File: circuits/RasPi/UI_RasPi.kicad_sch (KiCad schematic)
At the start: 14 parts, among them Q30 BSS138, Q33 BSS138

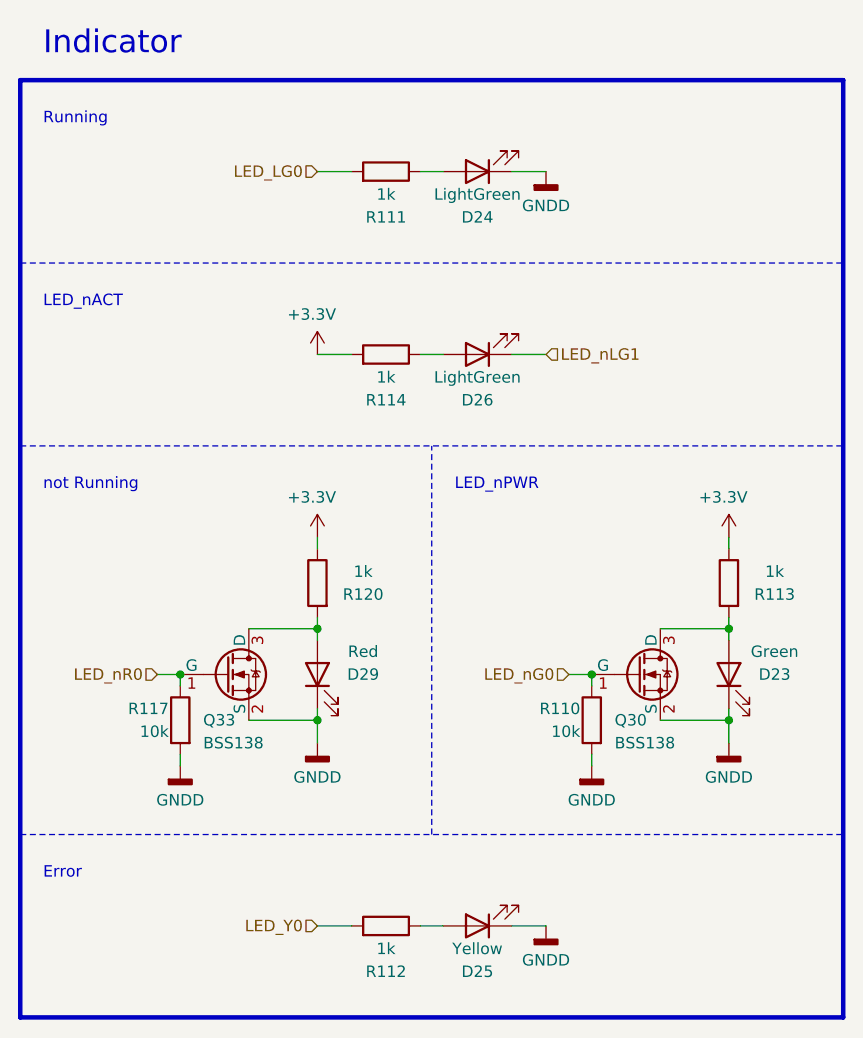
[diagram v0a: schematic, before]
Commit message: 更新
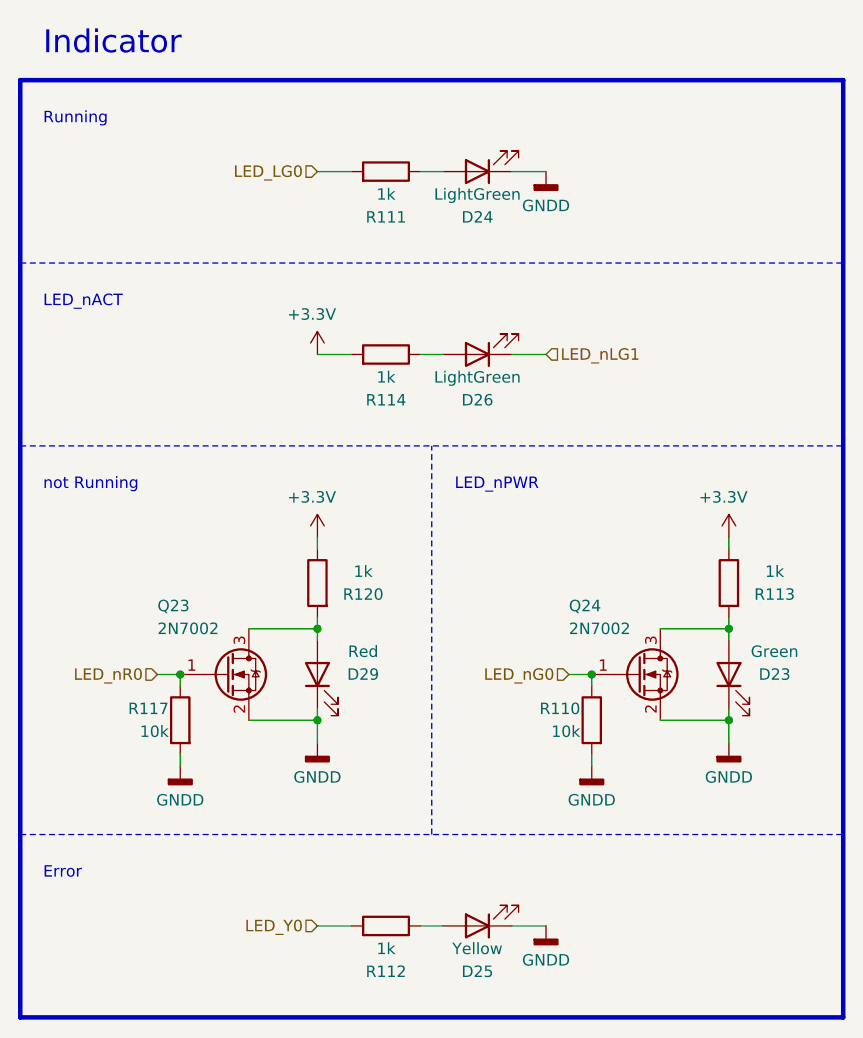
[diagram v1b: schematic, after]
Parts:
- removed Q30, Q33: BSS138, Package_TO_SOT_SMD:SOT-23, symbol Device:Q_NMOS_GSD
- added Q23, Q24: 2N7002, Package_TO_SOT_SMD:SOT-23, symbol Transistor_FET:2N7002
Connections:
- net GNDD: now also Q23.2 (S), Q24.2 (S)
- net LED_nG0: now also Q24.1 (G)
- net LED_nR0: now also Q23.1 (G)
- net at D23.2 (A), R113.2: now also Q24.3 (D)
- net at D29.2 (A), R120.2: now also Q23.3 (D)
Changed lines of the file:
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@@
   (junction (at 147.32 106.68) (diameter 0) (color 0 0 0 0)
   )
+  (junction (at 132.08 111.76) (diameter 0) (color 0 0 0 0)
+  )
+  (junction (at 147.32 116.84) (diameter 0) (color 0 0 0 0)
+  )
   (junction (at 177.8 111.76) (diameter 0) (color 0 0 0 0)
-  )
-  (junction (at 147.32 116.84) (diameter 0) (color 0 0 0 0)
-  )
-  (junction (at 132.08 111.76) (diameter 0) (color 0 0 0 0)
   )
   (junction (at 193.04 116.84) (diameter 0) (color 0 0 0 0)
@@
     )
   )
+  (symbol (lib_id "Transistor_FET:2N7002") (at 137.16 111.76 0) (unit 1)
+    (in_bom yes) (on_board yes) (dnp no)
+    (property "Reference" "Q23" (at 129.54 104.14 0)
+      (effects (font (size 1.27 1.27)) (justify left))
+    )
+    (property "Value" "2N7002" (at 129.54 106.68 0)
+      (effects (font (size 1.27 1.27)) (justify left))
+    )
+    (property "Footprint" "Package_TO_SOT_SMD:SOT-23" (at 142.24 113.665 0)
+      (effects (font (size 1.27 1.27) italic) (justify left) hide)
+    )
+    (property "Datasheet" "https://www.onsemi.com/pub/Collateral/NDS7002A-D.PDF" (at 142.24 115.57 0)
+      (effects (font (size 1.27 1.27)) (justify left) hide)
+    )
+    (pin "3")
+    (pin "1")
+    (pin "2")
+    (instances
+      (project "RasPi"
+        (path "/689a9e74-f202-4ea4-bfbb-4341f2549250/fddad0c3-2af8-46e3-8794-fa1122d24d51/69fce92a-28f6-4191-9f2f-418081756bee"
+          (reference "Q23") (unit 1)
+        )
+      )
+    )
+  )
   (symbol (lib_id "Device:LED") (at 193.04 111.76 90) (unit 1)
     (in_bom yes) (on_board yes) (dnp no)
@@
         (path "/689a9e74-f202-4ea4-bfbb-4341f2549250/fddad0c3-2af8-46e3-8794-fa1122d24d51/69fce92a-28f6-4191-9f2f-418081756bee"
           (reference "R120") (unit 1)
-        )
-      )
-    )
-  )
-  (symbol (lib_name "Q_NMOS_GSD_1") (lib_id "Device:Q_NMOS_GSD") (at 182.88 111.76 0) (unit 1)
-    (in_bom yes) (on_board yes) (dnp no)
-    (property "Reference" "Q30" (at 180.34 116.84 0)
-      (effects (font (size 1.27 1.27)) (justify left))
-    )
-    (property "Value" "BSS138" (at 180.34 119.38 0)
-      (effects (font (size 1.27 1.27)) (justify left))
-    )
-    (property "Footprint" "Package_TO_SOT_SMD:SOT-23" (at 187.96 109.22 0)
-      (effects (font (size 1.27 1.27)) hide)
-    )
-    (property "Datasheet" "~" (at 182.88 111.76 0)
-      (effects (font (size 1.27 1.27)) hide)
-    )
-    (pin "1")
-    (pin "2")
-    (pin "3")
-    (instances
-      (project "RasPi"
-        (path "/689a9e74-f202-4ea4-bfbb-4341f2549250/fddad0c3-2af8-46e3-8794-fa1122d24d51/69fce92a-28f6-4191-9f2f-418081756bee"
-          (reference "Q30") (unit 1)
         )
       )
@@
     )
   )
+  (symbol (lib_id "Transistor_FET:2N7002") (at 182.88 111.76 0) (unit 1)
+    (in_bom yes) (on_board yes) (dnp no)
+    (property "Reference" "Q24" (at 175.26 104.14 0)
+      (effects (font (size 1.27 1.27)) (justify left))
+    )
+    (property "Value" "2N7002" (at 175.26 106.68 0)
+      (effects (font (size 1.27 1.27)) (justify left))
+    )
+    (property "Footprint" "Package_TO_SOT_SMD:SOT-23" (at 187.96 113.665 0)
+      (effects (font (size 1.27 1.27) italic) (justify left) hide)
+    )
+    (property "Datasheet" "https://www.onsemi.com/pub/Collateral/NDS7002A-D.PDF" (at 187.96 115.57 0)
+      (effects (font (size 1.27 1.27)) (justify left) hide)
+    )
+    (pin "3")
+    (pin "1")
+    (pin "2")
+    (instances
+      (project "RasPi"
+        (path "/689a9e74-f202-4ea4-bfbb-4341f2549250/fddad0c3-2af8-46e3-8794-fa1122d24d51/69fce92a-28f6-4191-9f2f-418081756bee"
+          (reference "Q24") (unit 1)
+        )
+      )
+    )
+  )
   (symbol (lib_id "Device:R") (at 154.94 139.7 270) (mirror x) (unit 1)
     (in_bom yes) (on_board yes) (dnp no)
@@
         )
       )
-    )
-  )
-  (symbol (lib_name "Q_NMOS_GSD_1") (lib_id "Device:Q_NMOS_GSD") (at 137.16 111.76 0) (unit 1)
-    (in_bom yes) (on_board yes) (dnp no)
-    (property "Reference" "Q33" (at 134.62 116.84 0)
-      (effects (font (size 1.27 1.27)) (justify left))
-    )
-    (property "Value" "BSS138" (at 134.62 119.38 0)
-      (effects (font (size 1.27 1.27)) (justify left))
-    )
-    (property "Footprint" "Package_TO_SOT_SMD:SOT-23" (at 142.24 109.22 0)
-      (effects (font (size 1.27 1.27)) hide)
-    )
-    (property "Datasheet" "~" (at 137.16 111.76 0)
-      (effects (font (size 1.27 1.27)) hide)
-    )
-    (pin "1")
-    (pin "2")
-    (pin "3")
-    (instances
-      (project "RasPi"
-        (path "/689a9e74-f202-4ea4-bfbb-4341f2549250/fddad0c3-2af8-46e3-8794-fa1122d24d51/69fce92a-28f6-4191-9f2f-418081756bee"
-          (reference "Q33") (unit 1)
-        )
-      )
